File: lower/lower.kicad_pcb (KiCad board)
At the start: 2 copper layers, 177.8 x 127 mm, 4 parts

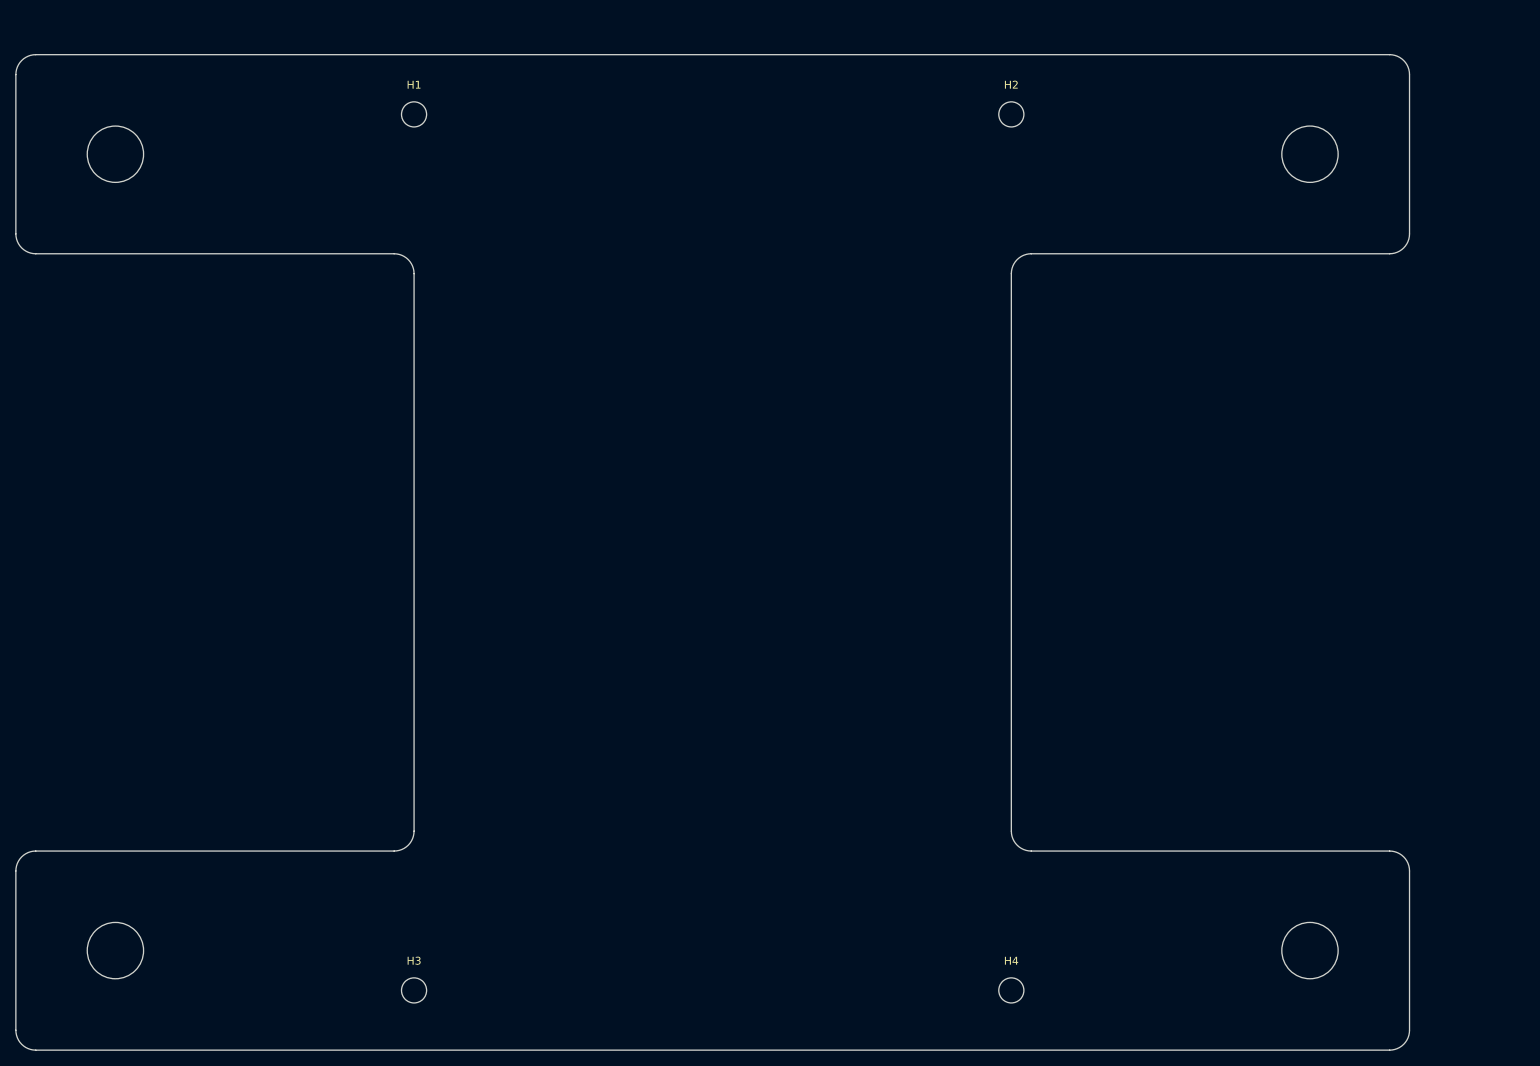
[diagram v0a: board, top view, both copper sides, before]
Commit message: Lower v0.1.0. Pre-routing
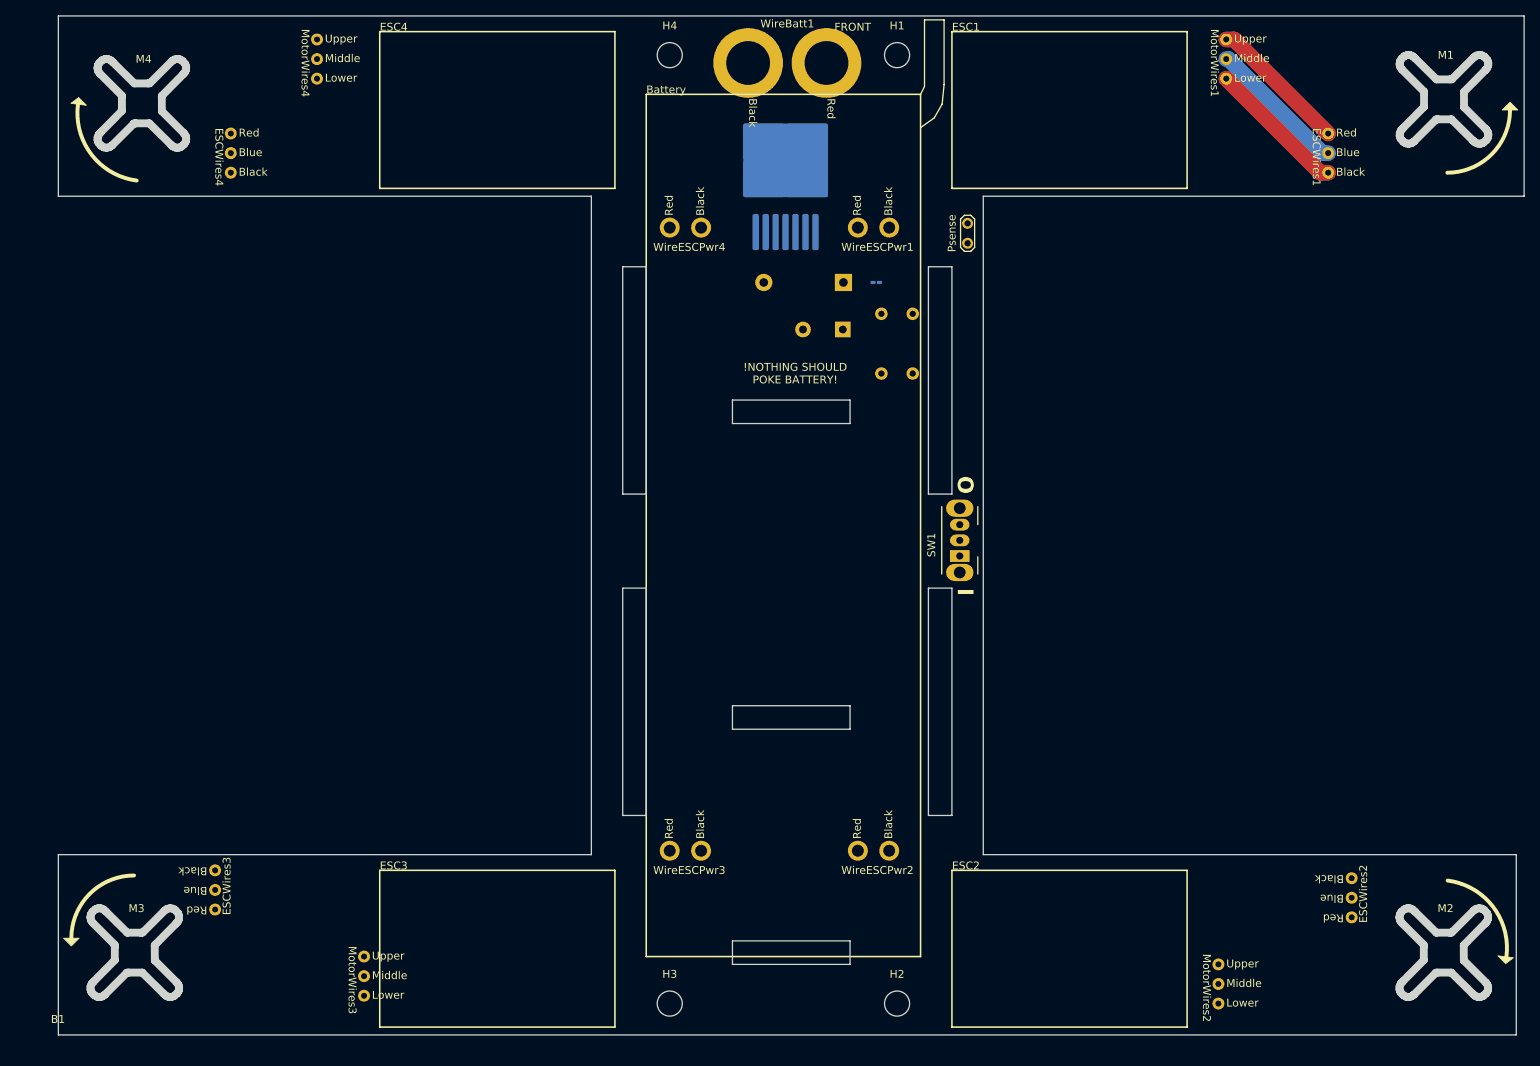
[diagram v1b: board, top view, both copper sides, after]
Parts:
- added B1: board-outline, lower-all:board-outline-test, F.Cu at (74.0, 153.0)
- added D1: 2.7V, Diode_THT:D_T-1_P5.08mm_Horizontal, B.Cu at (174.1, 63.0)
- added D2: 1N4007, Diode_THT:D_DO-41_SOD81_P10.16mm_Horizontal, B.Cu at (174.2, 57.0)
- added ESCWires1: ~, lower-all:WireESC, F.Cu at (236.0, 40.5)
- added ESCWires2: ~, lower-all:WireESC, F.Cu at (239.0, 135.5)
- added ESCWires3: ~, lower-all:WireESC, F.Cu at (94.0, 134.5)
- added ESCWires4: ~, lower-all:WireESC, F.Cu at (96.0, 40.5)
- added M1: MotorCutout, lower-all:MotorEdges, F.Cu at (250.5, 34.0)
- added M2: MotorCutout, lower-all:MotorEdges, F.Cu at (250.5, 142.9)
- added M3: MotorCutout, lower-all:MotorEdges, F.Cu at (83.5, 142.9)
- added M4: MotorCutout, lower-all:MotorEdges, F.Cu at (84.4, 34.5)
- added MotorWires1: ~, lower-all:WireMotor, F.Cu at (223.0, 28.5)
- added MotorWires2: ~, lower-all:WireMotor, F.Cu at (222.0, 146.5)
- added MotorWires3: ~, lower-all:WireMotor, F.Cu at (113.0, 145.5)
- added MotorWires4: ~, lower-all:WireMotor, F.Cu at (107.0, 28.5)
- added R1: 510, Resistor_SMD:R_0201_0603Metric_Pad0.64x0.40mm_HandSolder, B.Cu at (178.3, 57.0)
- added R2: 33, Resistor_THT:R_Axial_DIN0207_L6.3mm_D2.5mm_P7.62mm_Horizontal, B.Cu at (179.0, 68.6)
- added R3: 470, Resistor_THT:R_Axial_DIN0207_L6.3mm_D2.5mm_P7.62mm_Horizontal, B.Cu at (183.0, 61.0)
- added SW1: SW_SPDT, Button_Switch_THT:SW_Slide_SPDT_Angled_CK_OS102011MA1Q, F.Cu at (189.0, 91.9)
- added TP1: Psense, TestPoint:TestPoint_2Pads_Pitch2.54mm_Drill0.8mm, F.Cu at (190.0, 49.5)
- added U1: BTS50080-1TMA, Package_TO_SOT_SMD:TO-263-7_TabPin4, B.Cu at (166.8, 42.9)
- added WireBatt1: ~, lower-all:WireBatt, F.Cu at (167.0, 29.0)
- added WireESCPwr1: ~, lower-all:WireESCPwr, F.Cu at (178.0, 50.0)
- added WireESCPwr2: ~, lower-all:WireESCPwr, F.Cu at (178.0, 129.5)
- added WireESCPwr3: ~, lower-all:WireESCPwr, F.Cu at (154.0, 129.5)
- added WireESCPwr4: ~, lower-all:WireESCPwr, F.Cu at (154.0, 50.0)
- H1, H2, H3, H4: value MountingHole_Pad -> MountingHole
- moved H4 127.0 mm to (152.0, 28.0)
- moved H2 114.4 mm to (181.0, 149.0)
- moved H1 62.1 mm to (181.0, 28.0)
- moved H3 32.7 mm to (152.0, 149.0)
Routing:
- net /C1: track 0.00 -> 18.0 mm
- net /B1: track 0.00 -> 18.0 mm
- net /A1: track 0.00 -> 18.0 mm
- net /Vbb: track 0.00 -> 2.83 mm
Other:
- board size 177.8 x 127 mm -> 187 x 130 mm
- board text added: "!NOTHING SHOULD POKE BATTERY!"
- board text added: "Battery"
- board text added: "ESC1"
- board text added: "ESC2"
- board text added: "ESC3"
- board text added: "ESC4"
- board text added: "FRONT"
- board text added: "I"
- board text added: "M1"
- board text added: "M2"
- board text added: "M3"
- board text added: "M4"
- board text added: "O"
